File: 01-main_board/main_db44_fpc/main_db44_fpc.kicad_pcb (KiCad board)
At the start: 2 copper layers, 1 part

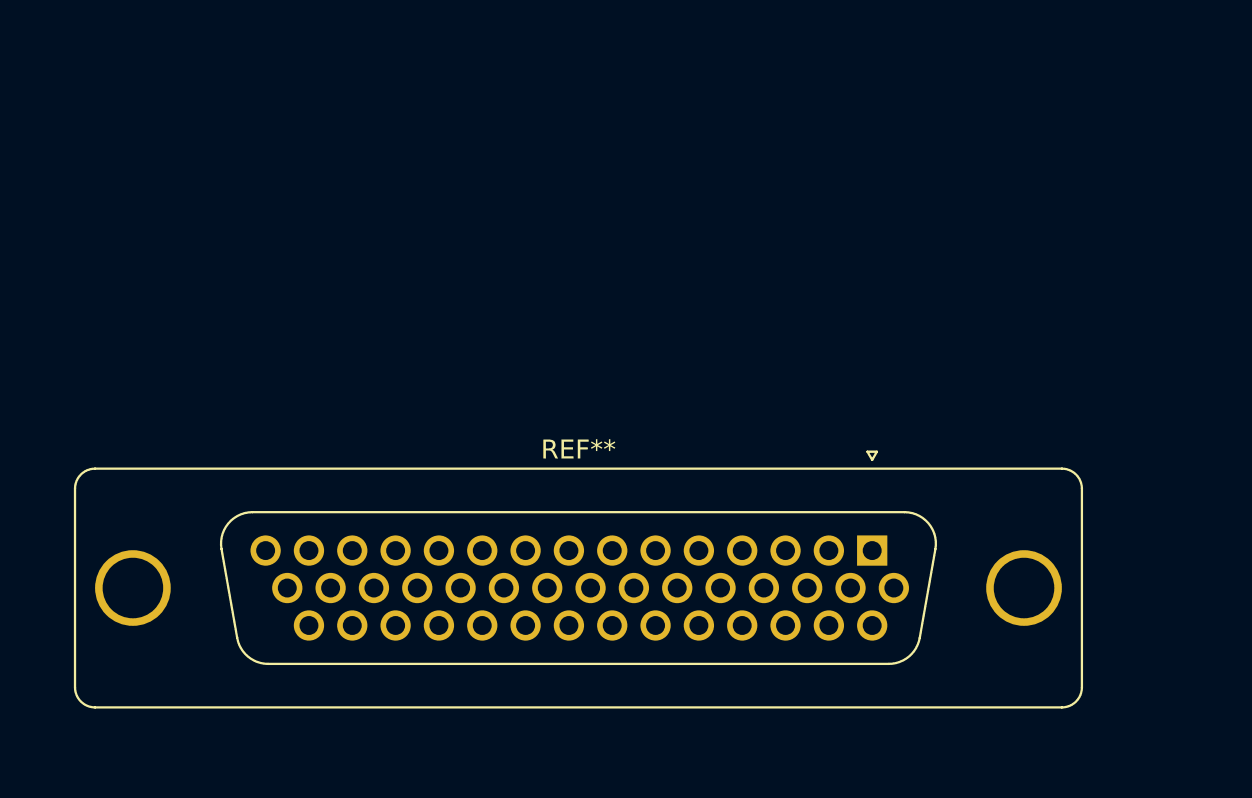
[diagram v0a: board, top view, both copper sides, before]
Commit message: update db44
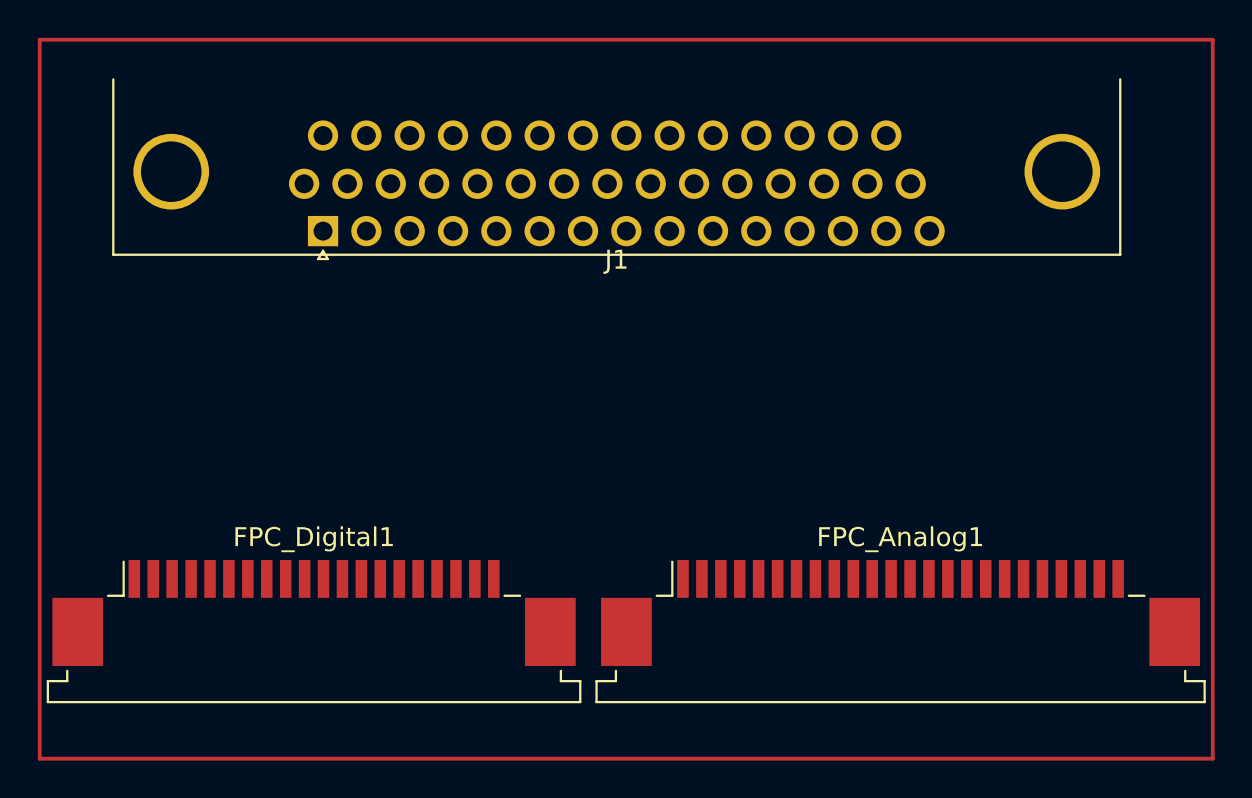
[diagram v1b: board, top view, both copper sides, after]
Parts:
- removed REF**: DSUB-44-HD_Socket_Vertical_P2.29x1.98mm_MountingHoles, Connector_Dsub:DSUB-44-HD_Socket_Vertical_P2.29x1.98mm_MountingHoles
- added FPC_Analog1: Conn_01x24, Connector_FFC-FPC:TE_2-84953-4_1x24-1MP_P1.0mm_Horizontal, F.Cu at (170.0, 101.8)
- added FPC_Digital1: Conn_01x20, Connector_FFC-FPC:TE_2-84953-0_1x20-1MP_P1.0mm_Horizontal, F.Cu at (139.0, 101.8)
- added J1: DB44_Female, jade_moon_footprints:female-DB44-TE-2311770-1-, F.Cu at (139.5, 80.4)
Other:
- copper layers 2 -> 4
